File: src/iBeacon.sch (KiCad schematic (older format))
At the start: 7 parts, among them IC1 AE-TYBLE16, P1 CONN_01X02, P2 CONN_01X02, P3 CONN_01X02

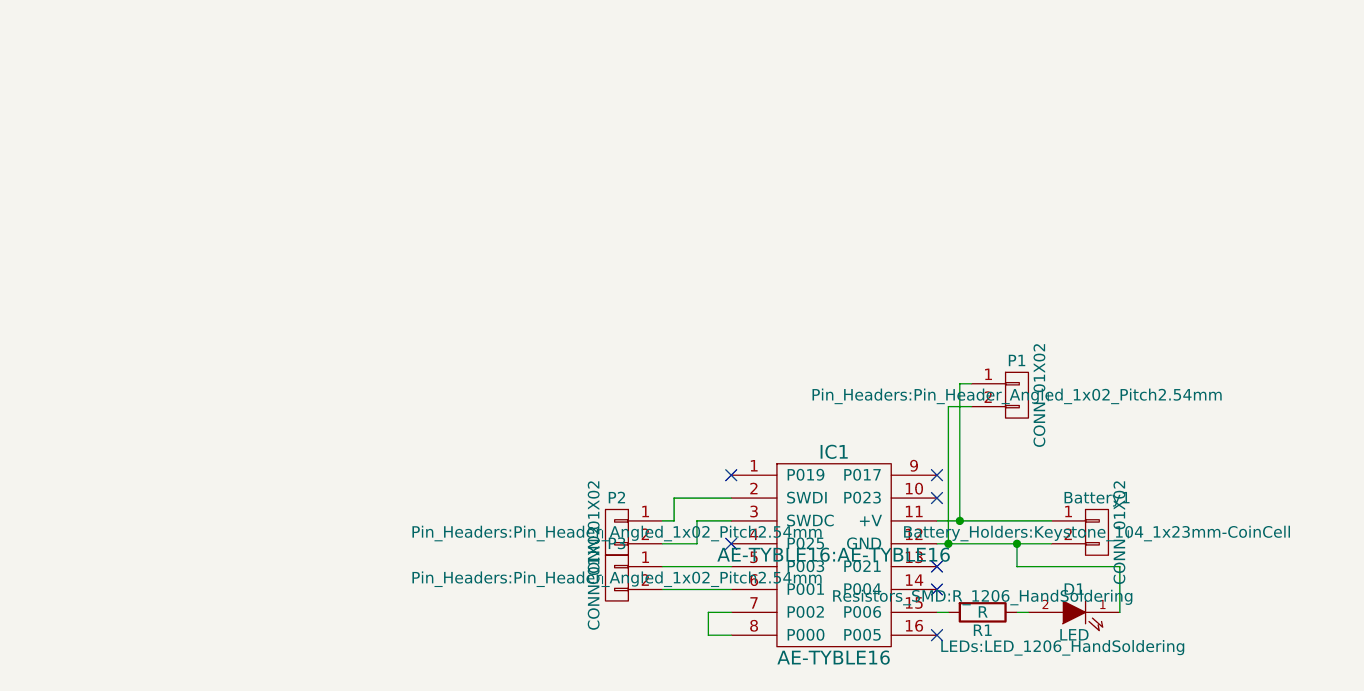
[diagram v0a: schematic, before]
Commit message: 2nd Version
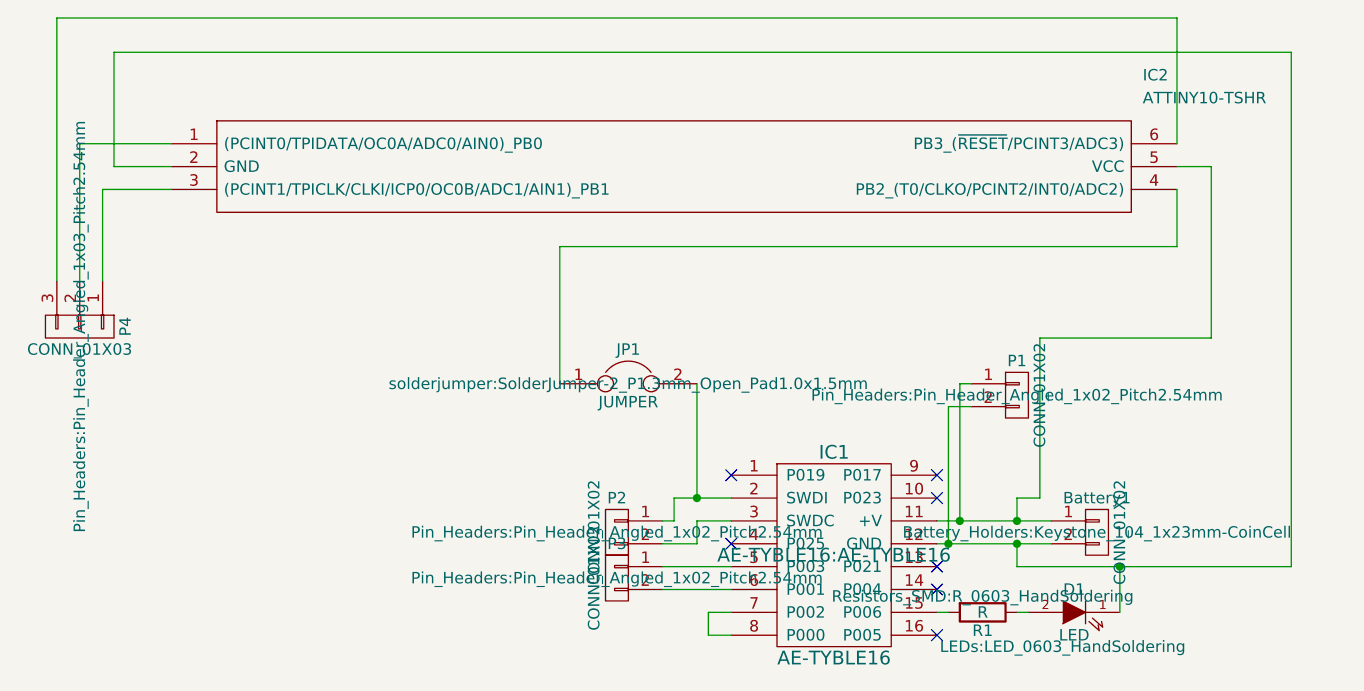
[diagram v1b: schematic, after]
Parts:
- added IC2: ATTINY10-TSHR, ATTINY10-TSHR:SOT95P280X145-6N, symbol ATTINY10-TSHR
- added JP1: JUMPER, solderjumper:SolderJumper-2_P1.3mm_Open_Pad1.0x1.5mm, symbol JUMPER
- added P4: CONN_01X03, Pin_Headers:Pin_Header_Angled_1x03_Pitch2.54mm, symbol CONN_01X03
- D1: footprint LEDs:LED_1206_HandSoldering -> LEDs:LED_0603_HandSoldering
- R1: footprint Resistors_SMD:R_1206_HandSoldering -> Resistors_SMD:R_0603_HandSoldering
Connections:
- net at Battery1.1 (P1), IC1.11 (+V), P1.1 (P1): now also IC2.5 (VCC)
- net at Battery1.2 (P2), D1.1 (K), IC1.12 (GND)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: now also IC2.2 (GND)
- net at IC1.2 (SWDI), P2.1 (P1): now also JP1.2
- new net: IC2.4 (PB2_(T0/CLKO/PCINT2/INT0/ADC2)), JP1.1
- new net: IC2.1 ((PCINT0/TPIDATA/OC0A/ADC0/AIN0)_PB0), P4.2 (P2)
- new net: IC2.3 ((PCINT1/TPICLK/CLKI/ICP0/OC0B/ADC1/AIN1)_PB1), P4.1 (P1)
- new net: IC2.6 (PB3_(~RESET~/PCINT3/ADC3)), P4.3 (P3)
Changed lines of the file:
@@
 LIBS:valves
 LIBS:ae-tyble16
+LIBS:ATTINY10-TSHR
 LIBS:iBeacon-cache
 EELAYER 25 0
@@
 NoConn ~ 5150 3300
 NoConn ~ 5150 3500
-Wire Wire Line
-	4250 3400 4150 3400
-Wire Wire Line
-	4150 3400 4150 3500
-Wire Wire Line
-	4150 3500 4250 3500
 $Comp
 L CONN_01X02 Battery1
@@
 	1    0    0    -1
 $EndComp
-Wire Wire Line
-	4250 3000 4100 3000
-Wire Wire Line
-	4100 3000 4100 3100
-Wire Wire Line
-	4100 3100 3950 3100
-Wire Wire Line
-	3950 3200 4250 3200
-Wire Wire Line
-	4250 3300 3950 3300
-Wire Wire Line
-	4000 2900 4250 2900
-Wire Wire Line
-	5150 3000 5650 3000
-Wire Wire Line
-	5150 3100 5650 3100
-Wire Wire Line
-	5300 2400 5250 2400
-Wire Wire Line
-	5250 2400 5250 3000
-Connection ~ 5250 3000
-Wire Wire Line
-	5300 2500 5200 2500
-Wire Wire Line
-	5200 2500 5200 3100
-Connection ~ 5200 3100
 $Comp
 L AE-TYBLE16 IC1
@@
 F 0 "R1" V 5430 3400 50  0000 C CNN
 F 1 "R" V 5350 3400 50  0000 C CNN
-F 2 "Resistors_SMD:R_1206_HandSoldering" V 5280 3400 50  0000 C CNN
+F 2 "Resistors_SMD:R_0603_HandSoldering" V 5280 3400 50  0000 C CNN
 F 3 "" H 5350 3400 50  0000 C CNN
 	1    5350 3400
@@
 F 0 "D1" H 5750 3500 50  0000 C CNN
 F 1 "LED" H 5750 3300 50  0000 C CNN
-F 2 "LEDs:LED_1206_HandSoldering" H 5800 3250 50  0000 C CNN
+F 2 "LEDs:LED_0603_HandSoldering" H 5800 3250 50  0000 C CNN
 F 3 "" H 5750 3400 50  0000 C CNN
 	1    5750 3400
 	-1   0    0    -1
 $EndComp
-Wire Wire Line
-	5150 3400 5200 3400
-Wire Wire Line
-	5500 3400 5550 3400
-Wire Wire Line
-	5950 3200 5950 3400
-Wire Wire Line
-	5500 3200 5950 3200
-Wire Wire Line
-	5500 3100 5500 3200
-Connection ~ 5500 3100
 $Comp
 L CONN_01X02 P3
@@
 	1    0    0    -1
 $EndComp
+$Comp
+L JUMPER JP1
+U 1 1 5CA0BF62
+P 3800 2400
+F 0 "JP1" H 3800 2550 50  0000 C CNN
+F 1 "JUMPER" H 3800 2320 50  0000 C CNN
+F 2 "solderjumper:SolderJumper-2_P1.3mm_Open_Pad1.0x1.5mm" H 3800 2400 50  0000 C CNN
+F 3 "" H 3800 2400 50  0000 C CNN
+	1    3800 2400
+	1    0    0    -1
+$EndComp
+$Comp
+L ATTINY10-TSHR IC2
+U 1 1 5CA0BFA7
+P 1800 1350
+F 0 "IC2" H 6050 1650 50  0000 L CNN
+F 1 "ATTINY10-TSHR" H 6050 1550 50  0000 L CNN
+F 2 "ATTINY10-TSHR:SOT95P280X145-6N" H 6050 1450 50  0001 L CNN
+F 3 "http://www.atmel.com/images/atmel-8127-avr-8-bit-microcontroller-attiny4-attiny5-attiny9-attiny10_datasheet.pdf" H 6050 1350 50  0001 L CNN
+F 4 "ATTINY10-TSHR, 8 bit AVR Microcontroller 12MHz 1024 B Flash, 32 B RAM, 6-Pin SOT-23" H 6050 1250 50  0001 L CNN "Description"
+F 5 "1.45" H 6050 1150 50  0001 L CNN "Height"
+F 6 "Microchip" H 6050 1050 50  0001 L CNN "Manufacturer_Name"
+F 7 "ATTINY10-TSHR" H 6050 950 50  0001 L CNN "Manufacturer_Part_Number"
+F 8 "556-ATTINY10-TSHR" H 6050 850 50  0001 L CNN "Mouser Part Number"
+F 9 "https://www.mouser.com/Search/Refine.aspx?Keyword=556-ATTINY10-TSHR" H 6050 750 50  0001 L CNN "Mouser Price/Stock"
+F 10 "1330946P" H 6050 650 50  0001 L CNN "RS Part Number"
+F 11 "http://uk.rs-online.com/web/p/products/1330946P" H 6050 550 50  0001 L CNN "RS Price/Stock"
+	1    1800 1350
+	1    0    0    -1
+$EndComp
+Wire Wire Line
+	4250 3400 4150 3400
+Wire Wire Line
+	4150 3400 4150 3500
+Wire Wire Line
+	4150 3500 4250 3500
+Wire Wire Line
+	4250 3000 4100 3000
+Wire Wire Line
+	4100 3000 4100 3100
+Wire Wire Line
+	4100 3100 3950 3100
+Wire Wire Line
+	3950 3200 4250 3200
+Wire Wire Line
+	4250 3300 3950 3300
+Wire Wire Line
+	4000 2900 4250 2900
+Wire Wire Line
+	5150 3000 5650 3000
+Wire Wire Line
+	5150 3100 5650 3100
+Wire Wire Line
+	5300 2400 5250 2400
+Wire Wire Line
+	5250 2400 5250 3000
+Connection ~ 5250 3000
+Wire Wire Line
+	5300 2500 5200 2500
+Wire Wire Line
+	5200 2500 5200 3100
+Connection ~ 5200 3100
+Wire Wire Line
+	5150 3400 5200 3400
+Wire Wire Line
+	5500 3400 5550 3400
+Wire Wire Line
+	5950 3200 5950 3400
+Wire Wire Line
+	5500 3200 6700 3200
+Wire Wire Line
+	5500 3100 5500 3200
+Connection ~ 5500 3100
 Wire Wire Line
 	4000 2900 4000 3000
 Wire Wire Line
 	4000 3000 3950 3000
+Wire Wire Line
+	4100 2400 4100 2900
+Connection ~ 4100 2900
+Wire Wire Line
+	3500 2400 3500 1800
+Wire Wire Line
+	3500 1800 6200 1800
+Wire Wire Line
+	6200 1800 6200 1550
+Wire Wire Line
+	6200 1450 6350 1450
+Wire Wire Line
+	6350 1450 6350 2200
+Wire Wire Line
+	6350 2200 5600 2200
+Wire Wire Line
+	5600 2200 5600 2900
+Wire Wire Line
+	5600 2900 5500 2900
+Wire Wire Line
+	5500 2900 5500 3000
+Connection ~ 5500 3000
+Wire Wire Line
+	6700 3200 6700 950
+Wire Wire Line
+	6700 950  1550 950
+Wire Wire Line
+	1550 950  1550 1450
+Wire Wire Line
+	1550 1450 1800 1450
+Connection ~ 5950 3200
+$Comp
+L CONN_01X03 P4
+U 1 1 5CA0C661
+P 1400 2150
+F 0 "P4" H 1400 2350 50  0000 C CNN
+F 1 "CONN_01X03" V 1500 2150 50  0000 C CNN
+F 2 "Pin_Headers:Pin_Header_Angled_1x03_Pitch2.54mm" H 1400 2150 50  0000 C CNN
+F 3 "" H 1400 2150 50  0000 C CNN
+	1    1400 2150
+	0    1    1    0
+$EndComp
+Wire Wire Line
+	1800 1350 1400 1350
+Wire Wire Line
+	1400 1350 1400 1950
+Wire Wire Line
+	1800 1550 1500 1550
+Wire Wire Line
+	1500 1550 1500 1950
+Wire Wire Line
+	6200 1350 6200 800
+Wire Wire Line
+	6200 800  1300 800
+Wire Wire Line
+	1300 800  1300 1950
 $EndSCHEMATC
